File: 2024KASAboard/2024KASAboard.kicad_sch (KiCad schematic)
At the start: 7 parts, among them J1 Conn_01x04_Pin, J2 GPS, J3 Conn_01x07_Pin, J4 Conn_01x10_Pin, U1 Pico, U2 BME280

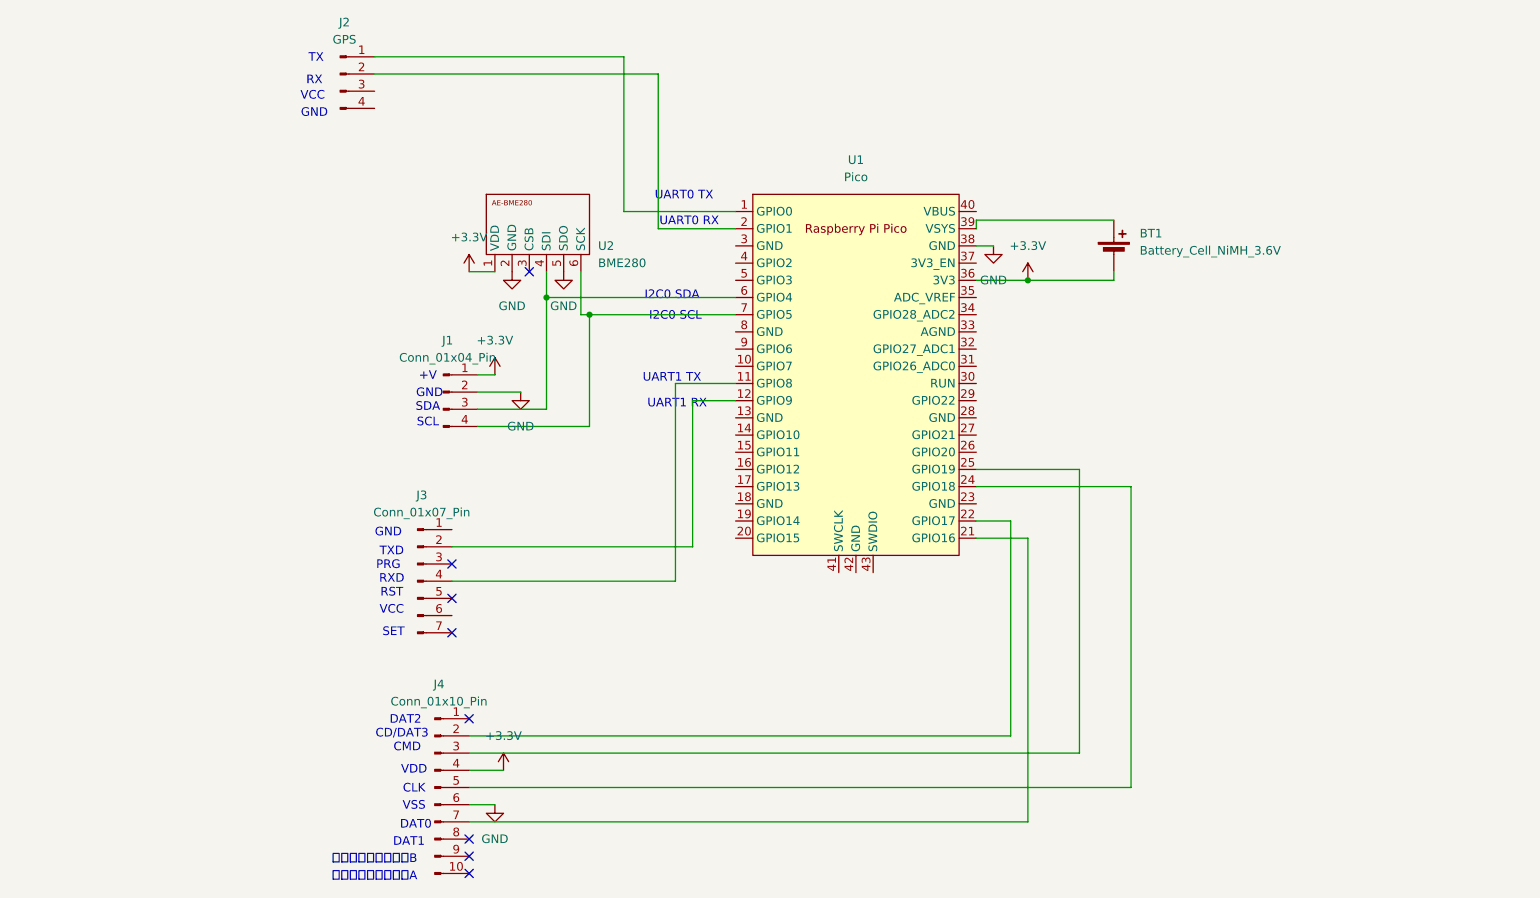
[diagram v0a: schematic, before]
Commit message: PCBdraft
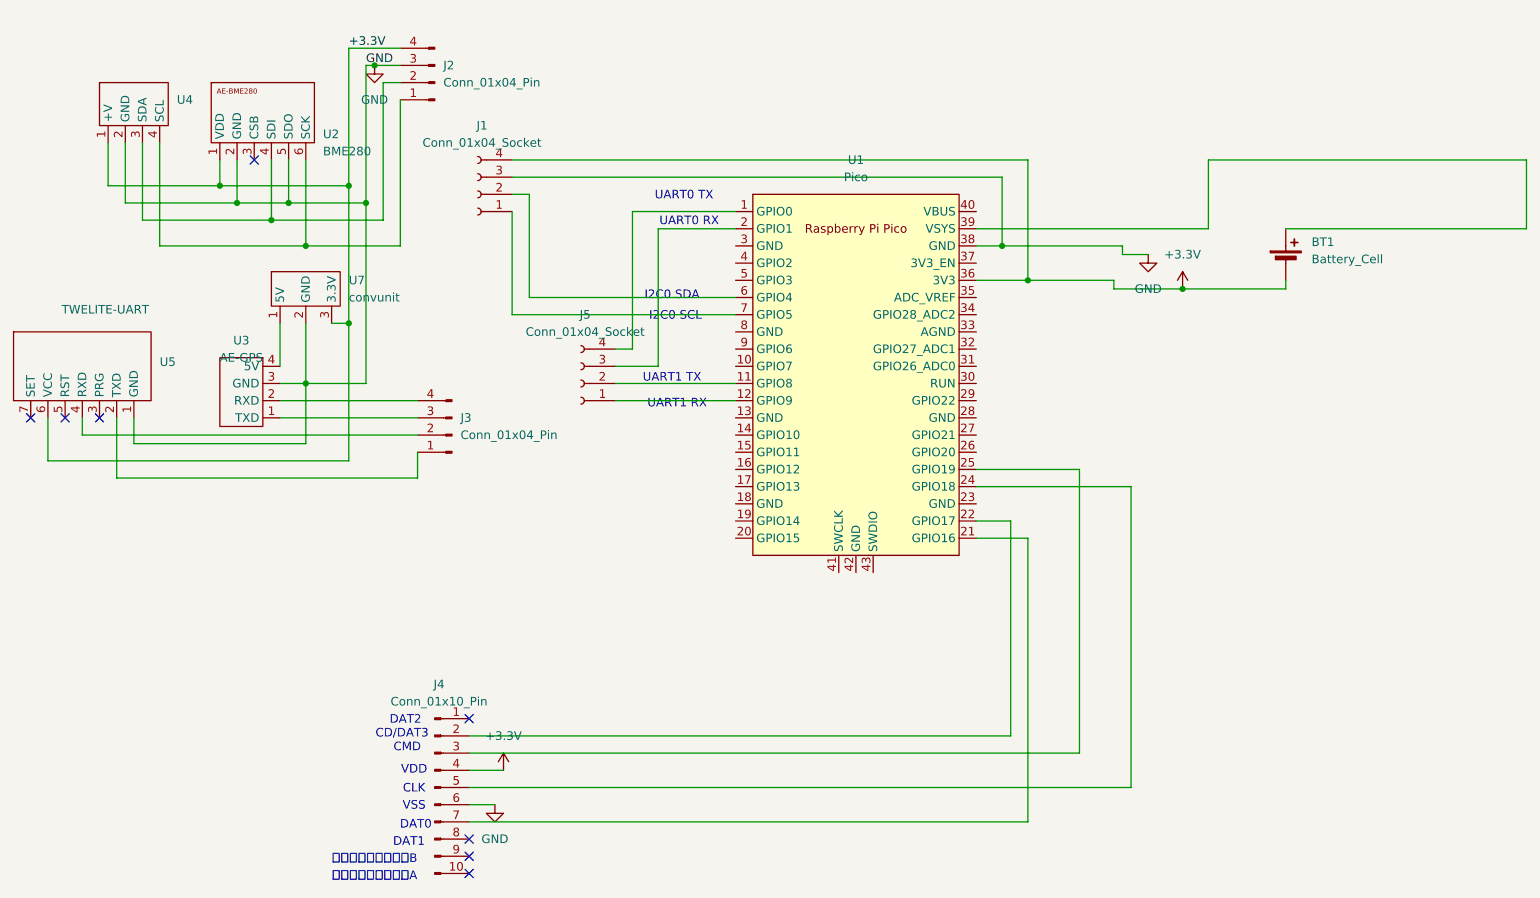
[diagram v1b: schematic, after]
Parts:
- removed J1: Conn_01x04_Pin, symbol Connector:Conn_01x04_Pin
- removed J3: Conn_01x07_Pin, symbol Connector:Conn_01x07_Pin
- added J1, J5: Conn_01x04_Socket, symbol Connector:Conn_01x04_Socket
- added J3: Conn_01x04_Pin, symbol Connector:Conn_01x04_Pin
- added U3: AE-GPS, symbol 0_kasa_lib-2024-:AE-GPS
- added U4: ~, symbol 0_kasa_lib-2024-:AE-LSM9DS1
- added U5: TWELITE-UART, symbol 0_kasa_lib-2024-:TWELITE-UART
- added U7: convunit, symbol 0_kasa_lib-2024-:convunit
- BT1: value Battery_Cell_NiMH_3.6V -> Battery_Cell
- J2: value GPS -> Conn_01x04_Pin
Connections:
- net +3.3V: now also J2.4 (Pin_4), J1.4 (Pin_4), U4.1 (+V), U5.6 (VCC), U7.3 (3.3V)
- net GND: now also J2.3 (Pin_3), J1.3 (Pin_3), U3.3 (GND), U4.2 (GND), U5.1 (GND), U7.2 (GND)
- net at U2.4 (SDI): now also J2.2 (Pin_2), U4.3 (SDA); no longer U1.6 (GPIO4)
- net at U2.6 (SCK): now also J2.1 (Pin_1), U4.4 (SCL); no longer U1.7 (GPIO5)
- net at U1.1 (GPIO0): now also J5.4 (Pin_4); no longer J2.1 (Pin_1)
- net at U1.2 (GPIO1): now also J5.3 (Pin_3); no longer J2.2 (Pin_2)
- net at U1.12 (GPIO9): now also J5.1 (Pin_1)
- net at U1.11 (GPIO8): now also J5.2 (Pin_2)
- new net: J3.1 (Pin_1), U5.2 (TXD)
- new net: J3.2 (Pin_2), U5.4 (RXD)
- new net: J3.3 (Pin_3), U3.1 (TXD)
- new net: J3.4 (Pin_4), U3.2 (RXD)
- new net: J1.1 (Pin_1), U1.7 (GPIO5)
- new net: J1.2 (Pin_2), U1.6 (GPIO4)
- new net: U3.4 (5V), U7.1 (5V)
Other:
- note removed: "+V"
- note removed: "GND"
- note removed: "PRG"
- note removed: "RST"
- note removed: "RX"
- note removed: "RXD"
- note removed: "SCL"
- note removed: "SDA"
- note removed: "SET"
- note removed: "TX"
- note removed: "TXD"
- note removed: "VCC"
- moved on the sheet: BT1, U2
